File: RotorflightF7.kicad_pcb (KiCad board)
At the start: 6 copper layers, 31 x 29 mm, 62 parts, among them J1 USB_C_Receptacle_USB2.0, J2 Outputs, J3 A, J4 DSM, J5 JTAG_TC2030, SW1 SW_Push, U1 ESD1014, U2 AP63205WU, U3 ESD1014, U4 USBLC6-2SC6, U5 XC6220B331MR, U6 STM32F722RETx, U7 BMI270, U8 SPL06-001, U9 W25N01G, Y1 8MHz

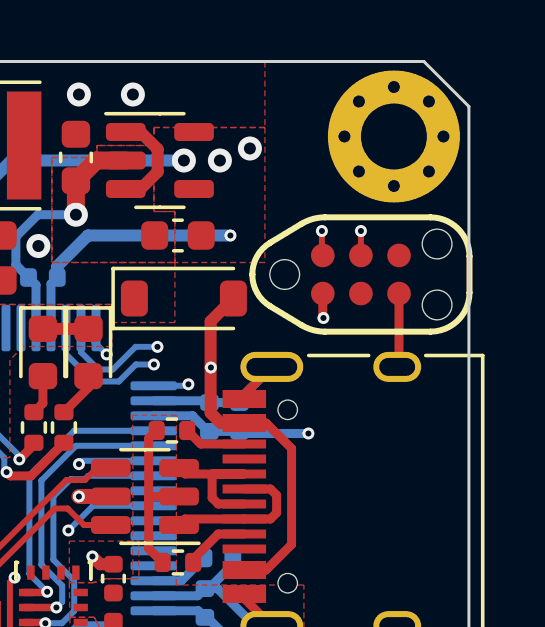
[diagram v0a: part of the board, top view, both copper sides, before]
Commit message: schematic visual updates
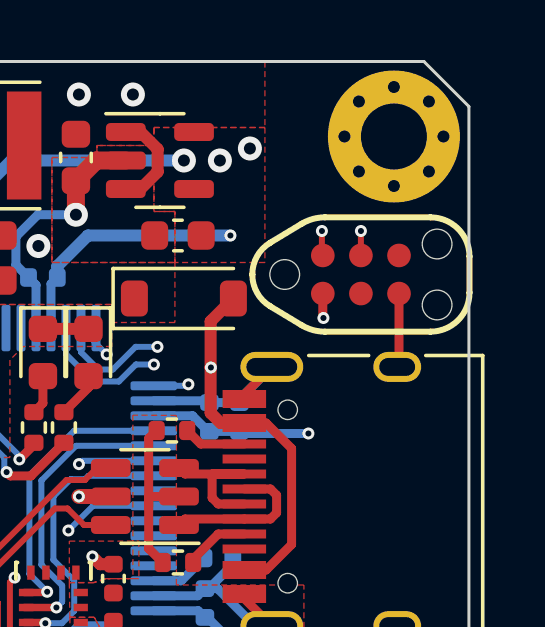
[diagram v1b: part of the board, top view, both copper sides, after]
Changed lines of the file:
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@@
         (effects (font (size 1 1) (thickness 0.15)))
     )
-    (fp_text value "Outputs" (at -2.54 20.11) (layer "F.Fab")
+    (fp_text value "Outputs" (at 10.1 12.6) (layer "F.Fab")
         (effects (font (size 1 1) (thickness 0.15)))
     )
@@
     (fp_arc (start 2.319501 -1.9055) (mid 3.23874 -1.524738) (end 3.6195 -0.605499)
       (stroke (width 0.2) (type solid)) (layer "F.SilkS"))
-    (fp_arc (start 3.6195 0.605498) (mid 3.238739 1.524738) (end 2.3195 1.9055)
+    (fp_arc (start 3.6195 0.605498) (mid 3.23874 1.524738) (end 2.3195 1.9055)
       (stroke (width 0.2) (type solid)) (layer "F.SilkS"))
     (fp_line (start -1.27 -0.635) (end 1.27 -0.635)
@@
     (polygon
       (pts
-        (xy 95.49 31.13)
-        (xy 134.49 31.13)
-        (xy 134.49 68.13)
-        (xy 95.49 68.13)
+        (xy 96.49 32.13)
+        (xy 132.49 32.13)
+        (xy 132.49 66.13)
+        (xy 96.49 66.13)
       )
     )
@@
     (polygon
       (pts
-        (xy 96.49 32.13)
-        (xy 133.99 32.13)
-        (xy 133.99 67.13)
-        (xy 96.49 67.13)
+        (xy 97.49 33.13)
+        (xy 131.49 33.13)
+        (xy 131.49 65.13)
+        (xy 97.49 65.13)
       )
     )
